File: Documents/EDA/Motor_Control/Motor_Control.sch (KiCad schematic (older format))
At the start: 8 parts, among them J1 V_MOTOR, M1 R, M2 Z

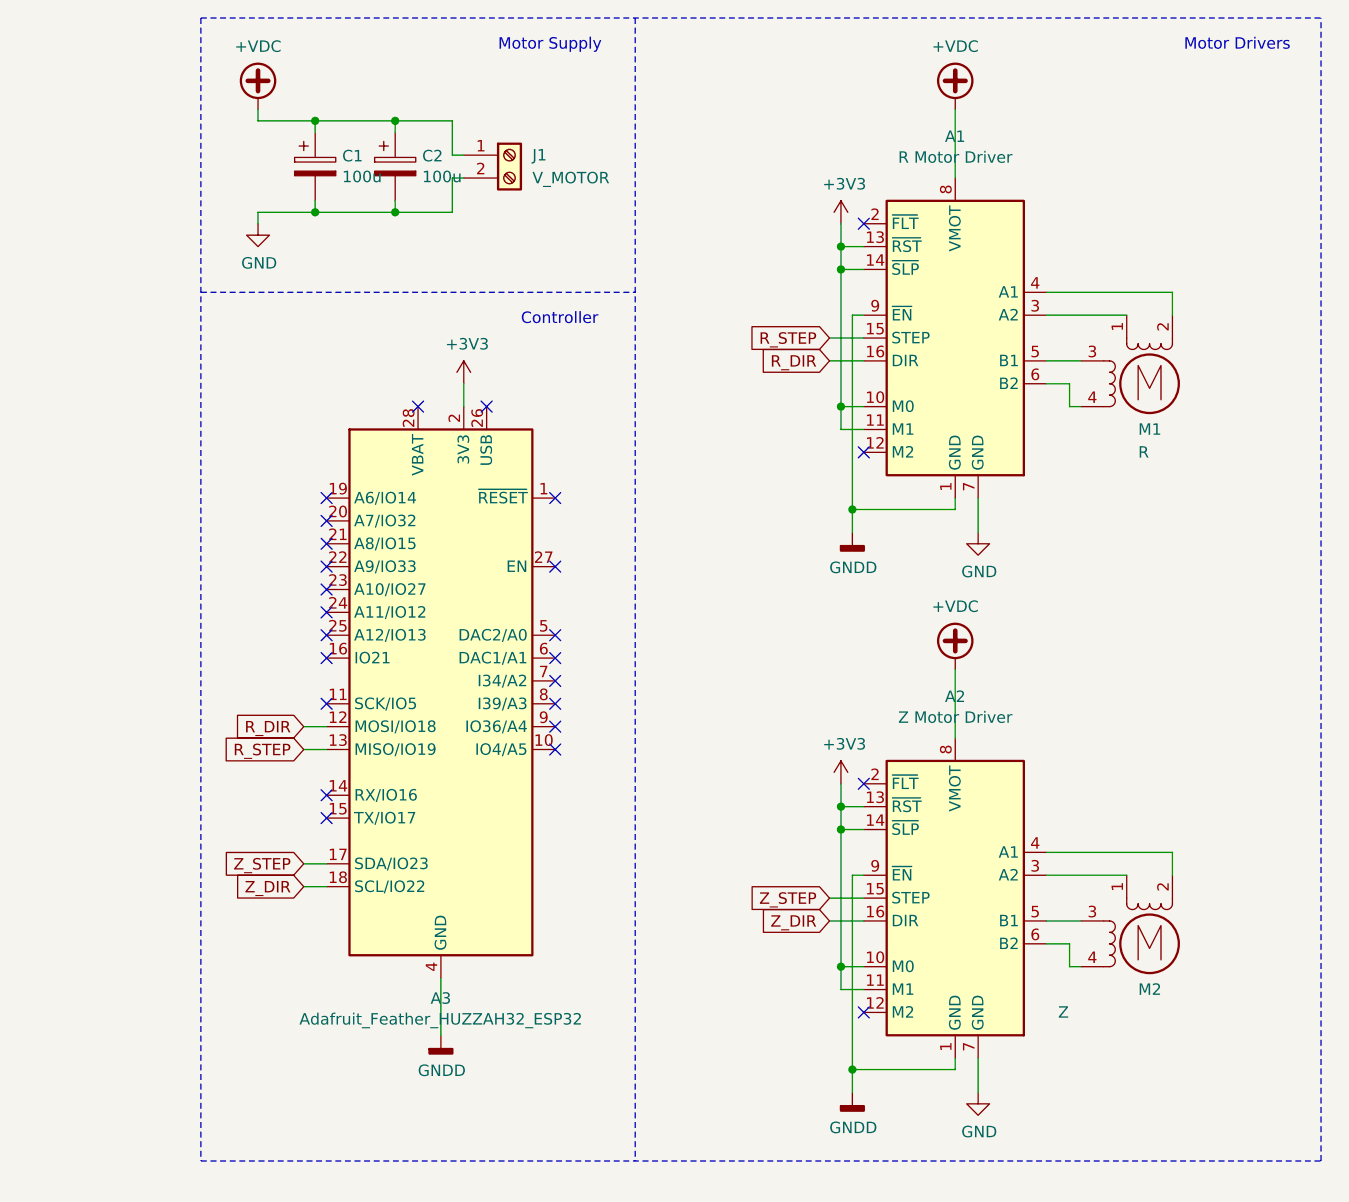
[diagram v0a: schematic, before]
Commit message: libs and pcb and bom
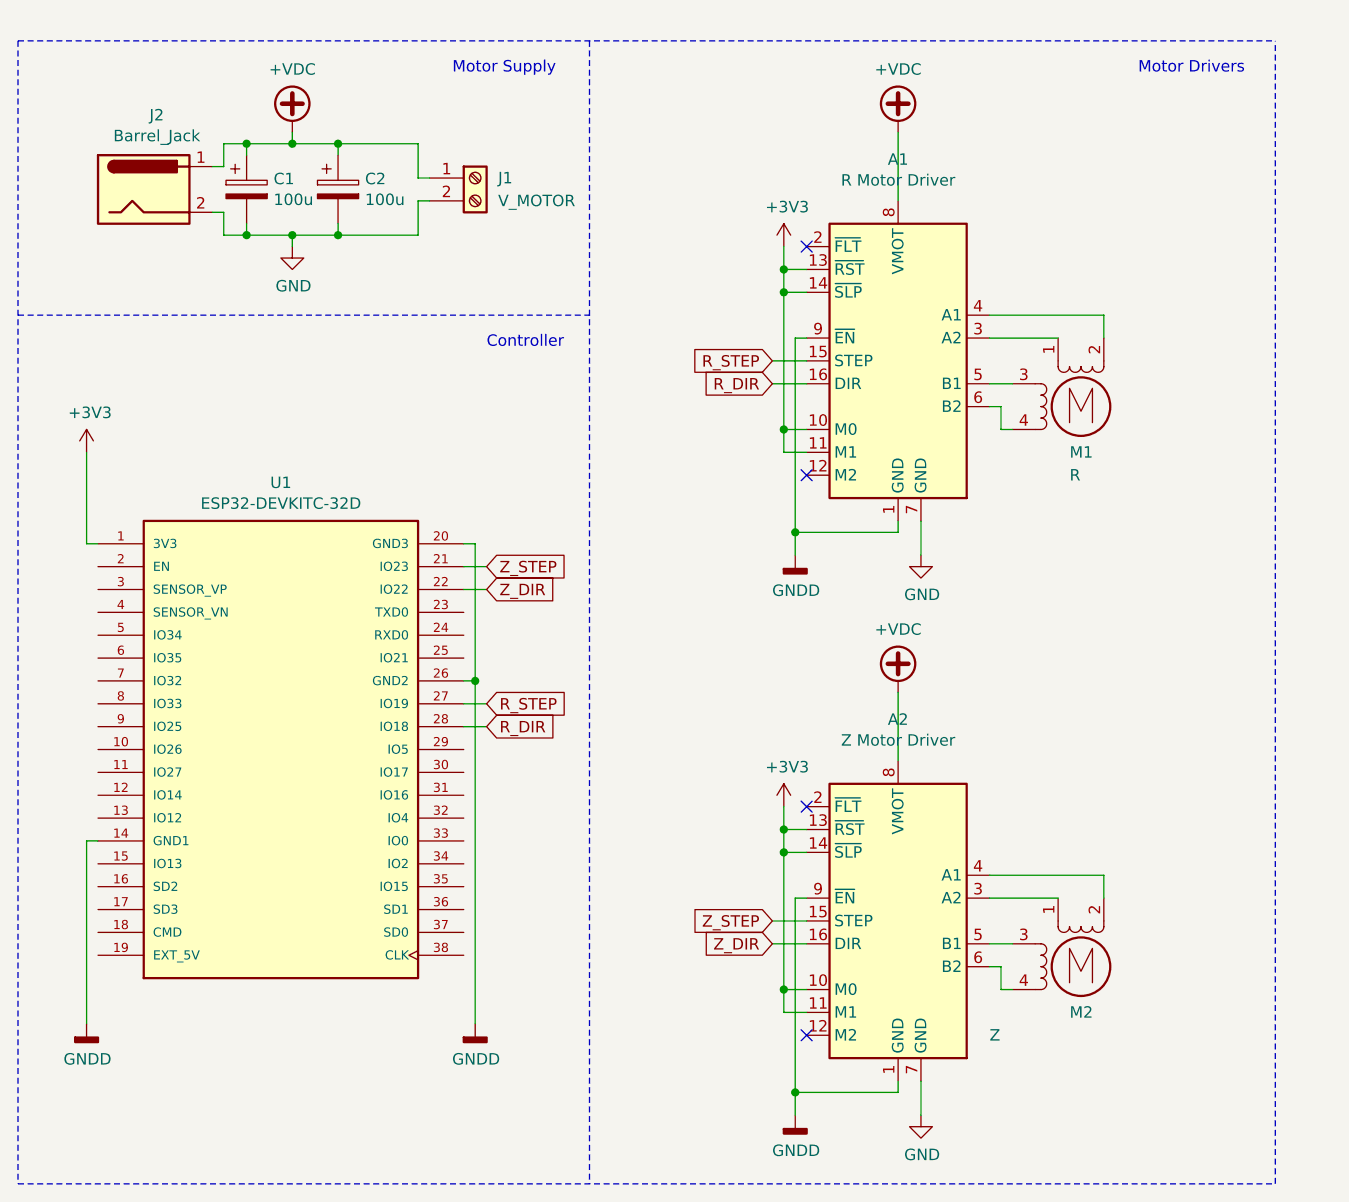
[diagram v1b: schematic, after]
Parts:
- removed A3: Adafruit_Feather_HUZZAH32_ESP32, Module:Adafruit_Feather, symbol MCU_Module:Adafruit_Feather_HUZZAH32_ESP32
- added J2: Barrel_Jack, Connector_BarrelJack:BarrelJack_Horizontal, symbol Connector:Barrel_Jack
- added U1: ESP32-DEVKITC-32D, MODULE_ESP32-DEVKITC-32D:MODULE_ESP32-DEVKITC-32D, symbol ESP32-DEVKITC-32D:ESP32-DEVKITC-32D
- M1, M2: footprint Connector_PinSocket_2.54mm:PinSocket_1x04_P2.54mm_Vertical -> (none)
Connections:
- net +3V3: now also U1.1 (3V3)
- net +VDC: now also J2.1
- net GND: now also J2.2
- net GNDD: now also U1.14 (GND1), U1.20 (GND3), U1.26 (GND2)
- net R_DIR: now also U1.28 (IO18)
- net R_STEP: now also U1.27 (IO19)
- net Z_DIR: now also U1.22 (IO22)
- net Z_STEP: now also U1.21 (IO23)
- no-connect marks 25 -> 4
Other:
- moved on the sheet: A1, A2, C1, C2, J1, M1, M2
